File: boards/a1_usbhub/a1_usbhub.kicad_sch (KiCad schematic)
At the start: 32 parts, among them U1 TXS0102DCT, U2 USB2517I-JZX, U3 AP62150Z6, U4 TPS2054D, U5 TPS2054D, U6 74LVC1G17

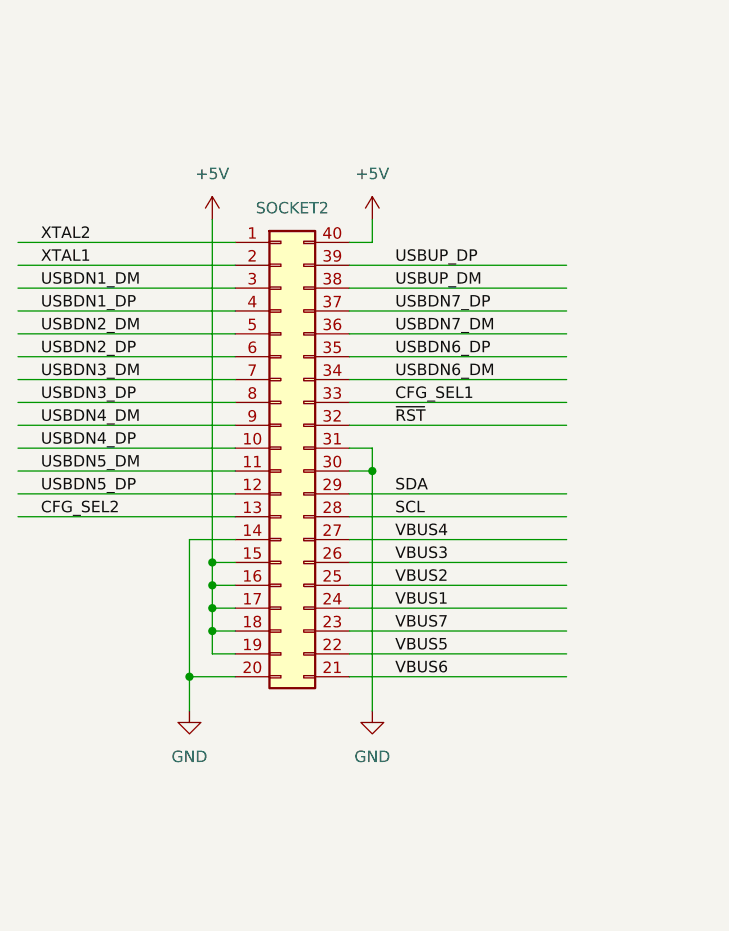
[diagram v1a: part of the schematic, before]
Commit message: USB HUB is back in.
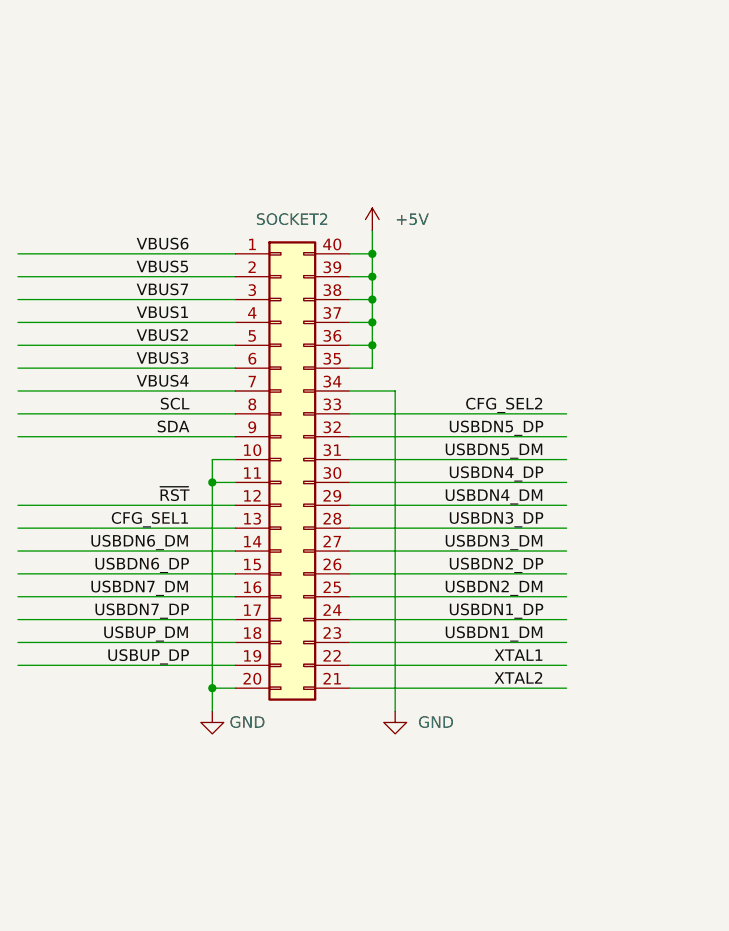
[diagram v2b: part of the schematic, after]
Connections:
- net +5V: now also SOCKET2.35 (Pin_35), SOCKET2.36 (Pin_36), SOCKET2.37 (Pin_37), SOCKET2.38 (Pin_38), SOCKET2.39 (Pin_39); no longer SOCKET2.15 (Pin_15), SOCKET2.16 (Pin_16), SOCKET2.17 (Pin_17), SOCKET2.18 (Pin_18), SOCKET2.19 (Pin_19)
- net CFG_SEL1: now also SOCKET2.13 (Pin_13); no longer SOCKET2.33 (Pin_33)
- net CFG_SEL2: now also SOCKET2.33 (Pin_33); no longer SOCKET2.13 (Pin_13)
- net GND: now also SOCKET2.10 (Pin_10), SOCKET2.11 (Pin_11), SOCKET2.34 (Pin_34); no longer SOCKET2.14 (Pin_14), SOCKET2.30 (Pin_30), SOCKET2.31 (Pin_31)
- net SCL: now also SOCKET2.8 (Pin_8); no longer SOCKET2.28 (Pin_28)
- net SDA: now also SOCKET2.9 (Pin_9); no longer SOCKET2.29 (Pin_29)
- net USBDN1_DM: now also SOCKET2.23 (Pin_23); no longer SOCKET2.3 (Pin_3)
- net USBDN1_DP: now also SOCKET2.24 (Pin_24); no longer SOCKET2.4 (Pin_4)
- net USBDN2_DM: now also SOCKET2.25 (Pin_25); no longer SOCKET2.5 (Pin_5)
- net USBDN2_DP: now also SOCKET2.26 (Pin_26); no longer SOCKET2.6 (Pin_6)
- net USBDN3_DM: now also SOCKET2.27 (Pin_27); no longer SOCKET2.7 (Pin_7)
- net USBDN3_DP: now also SOCKET2.28 (Pin_28); no longer SOCKET2.8 (Pin_8)
- net USBDN4_DM: now also SOCKET2.29 (Pin_29); no longer SOCKET2.9 (Pin_9)
- net USBDN4_DP: now also SOCKET2.30 (Pin_30); no longer SOCKET2.10 (Pin_10)
- net USBDN5_DM: now also SOCKET2.31 (Pin_31); no longer SOCKET2.11 (Pin_11)
- net USBDN5_DP: now also SOCKET2.32 (Pin_32); no longer SOCKET2.12 (Pin_12)
- net USBDN6_DM: now also SOCKET2.14 (Pin_14); no longer SOCKET2.34 (Pin_34)
- net USBDN6_DP: now also SOCKET2.15 (Pin_15); no longer SOCKET2.35 (Pin_35)
- net USBDN7_DM: now also SOCKET2.16 (Pin_16); no longer SOCKET2.36 (Pin_36)
- net USBDN7_DP: now also SOCKET2.17 (Pin_17); no longer SOCKET2.37 (Pin_37)
- net USBUP_DM: now also SOCKET2.18 (Pin_18); no longer SOCKET2.38 (Pin_38)
- net USBUP_DP: now also SOCKET2.19 (Pin_19); no longer SOCKET2.39 (Pin_39)
- net VBUS1: now also SOCKET2.4 (Pin_4); no longer SOCKET2.24 (Pin_24)
- net VBUS2: now also SOCKET2.5 (Pin_5); no longer SOCKET2.25 (Pin_25)
- net VBUS3: now also SOCKET2.6 (Pin_6); no longer SOCKET2.26 (Pin_26)
- net VBUS4: now also SOCKET2.7 (Pin_7); no longer SOCKET2.27 (Pin_27)
- net VBUS5: now also SOCKET2.2 (Pin_2); no longer SOCKET2.22 (Pin_22)
- net VBUS6: now also SOCKET2.1 (Pin_1); no longer SOCKET2.21 (Pin_21)
- net VBUS7: now also SOCKET2.3 (Pin_3); no longer SOCKET2.23 (Pin_23)
- net XTAL1: now also SOCKET2.22 (Pin_22); no longer SOCKET2.2 (Pin_2)
- net XTAL2: now also SOCKET2.21 (Pin_21); no longer SOCKET2.1 (Pin_1)
- net ~{RST}: now also SOCKET2.12 (Pin_12); no longer SOCKET2.32 (Pin_32)
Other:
- moved on the sheet: SOCKET2
